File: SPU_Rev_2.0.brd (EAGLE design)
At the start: 141 x 101.6 mm, 139 parts, among them Q1 12MHz

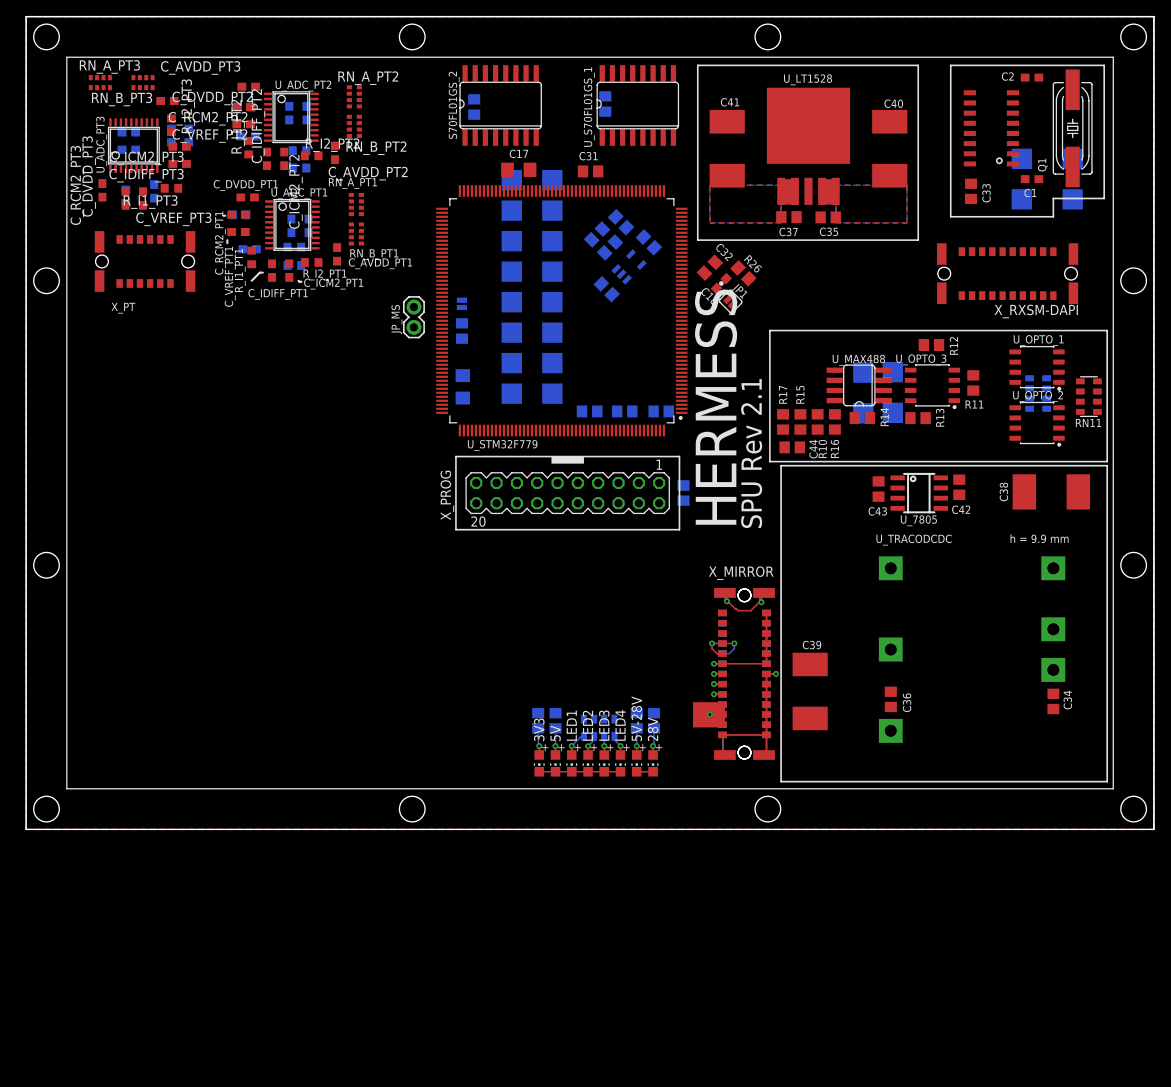
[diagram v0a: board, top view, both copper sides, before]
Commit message: rev 2.1
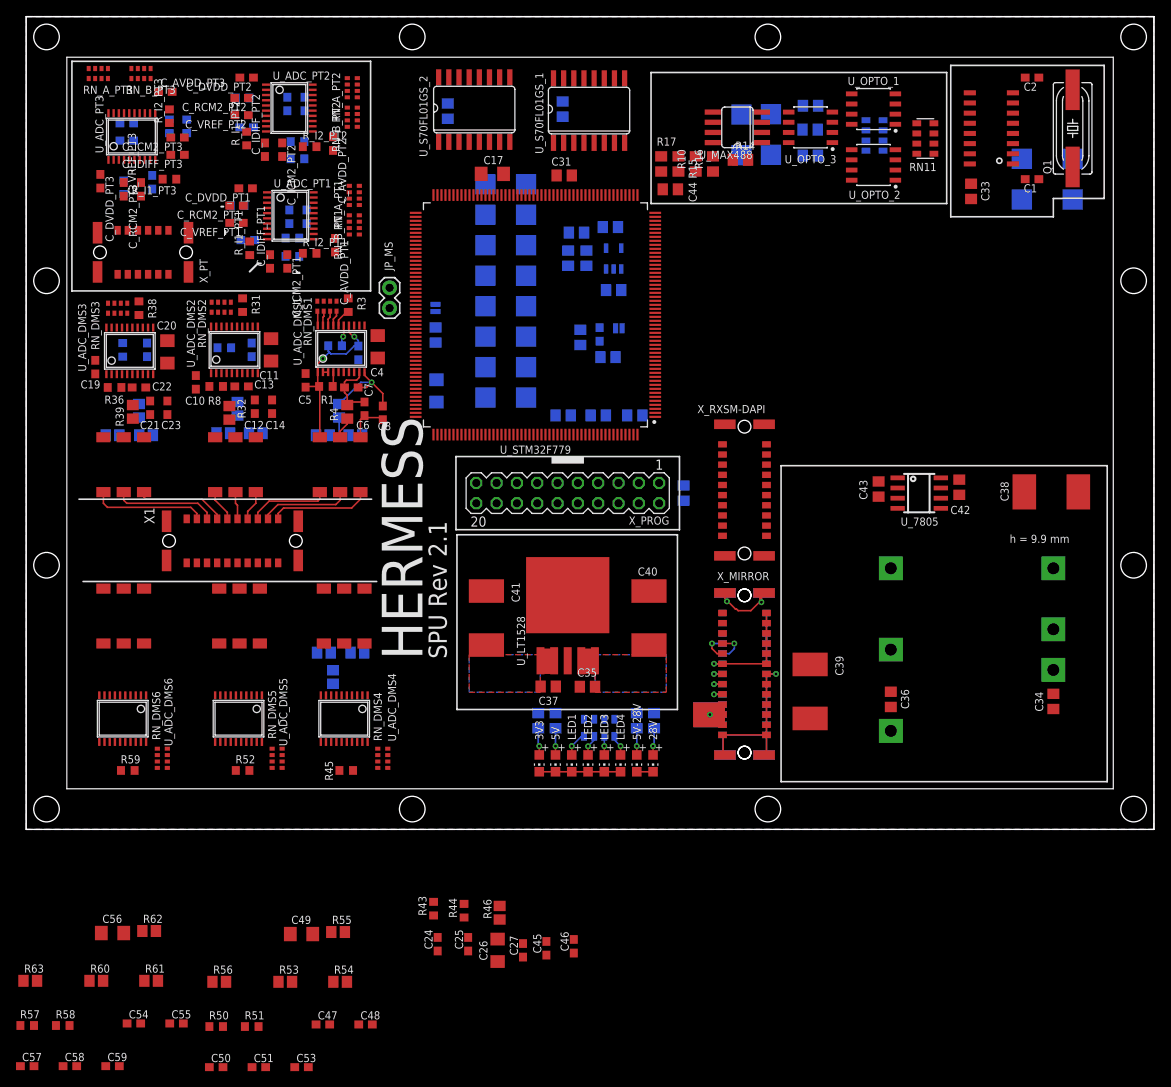
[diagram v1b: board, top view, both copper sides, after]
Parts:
- removed S70FL01GS_2: S70FL01GS, S70FL01GS:SO16
- added C10, C12, C13, C14, C15, C19, C21, C22, C23, C24, C25, C27, C3, C45, C46, C47, C48, C5, C50, C51, C53, C54, C55, C57, C58, C59, C6, C7, C8, C9: 100n, rcl:C0603
- added C11, C20, C26, C4, C49, C56: 1u, rcl:C1206
- added R1, R2, R30, R36, R37, R43, R44, R50, R51, R57, R58, R8: 4k7, ++Bedrahtet:R0603
- added R3, R31, R38, R45, R52, R59: 47, ++Bedrahtet:R0603
- added R32, R33, R39, R4, R40, R46, R47, R5, R53, R54, R60, R61: 40 1%, ++Bedrahtet:R0805
- added R34, R35, R41, R42, R48, R49, R55, R56, R6, R62, R63, R7: 1k 0.1%, ++Bedrahtet:R0805
- added RN_DMS1, RN_DMS2, RN_DMS3, RN_DMS4, RN_DMS5, RN_DMS6: 47, resistor-dil:0603-ARC
- added U$1, U$2, U$3, U$4, U$5, U$6: COMMON_MODE_CHOKE, selfmade:COMMON_MODE_CHOKE
- added U_ADC_DMS1, U_ADC_DMS2, U_ADC_DMS3, U_ADC_DMS4, U_ADC_DMS5, U_ADC_DMS6: ADS1147TSSOP20, ads11xx:TSSOP20
- added U_S70FL01GS_2: S70FL01GS, S70FL01GS:SO16
- added X1: 403-5X020-5X, con-ept-One27:403-5X020-5X
- moved C40 65.9 mm to (82.9, 26.4)
- moved C41 65.9 mm to (62.6, 26.4)
- moved C35 65.9 mm to (75.2, 17.8)
- moved C37 65.9 mm to (70.3, 17.9)
- moved U_LT1528 65.9 mm to (72.8, 29.0)
- moved X_RXSM-DAPI 42.6 mm to (94.9, 42.4), turned to 270 degrees
- moved RN11 38.2 mm to (117.5, 86.4)
- moved RN12 38.2 mm to (111.1, 86.7)
- moved U_OPTO_1 38.2 mm to (111.0, 90.0)
- moved U_OPTO_2 38.2 mm to (111.0, 83.1)
- moved R11 37.7 mm to (103.1, 87.5), flipped to the bottom, turned to 180 degrees
- moved R10 35.7 mm to (88.8, 83.2)
- moved U_OPTO_3 35.7 mm to (103.1, 87.8)
- moved C44 35.7 mm to (85.6, 80.0)
- moved D5 35.7 mm to (98.2, 86.9)
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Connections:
- net PT1_DIN renamed PT_DIN
- net PT1_DOUT renamed PT_DOUT
- net PT1_SCLK renamed PT_SCLK
- removed net PT1_!CS: RN_B_PT1.7, RN_B_PT2.7, RN_B_PT3.7
- removed net PT1_!DRDY: RN_B_PT1.8, RN_B_PT2.8, RN_B_PT3.8
- removed net PT1_!RESET: RN_A_PT1.8, RN_A_PT2.8, RN_A_PT3.8
- removed net PT1_START: RN_B_PT1.6, RN_B_PT2.6, RN_B_PT3.6
- new net !CS!_DMS1: R3.2
- new net !CS!_DMS2: R31.2
- new net !CS!_DMS3: R38.2
- new net !CS!_DMS4: R45.2
- new net !CS!_DMS5: R52.2
- new net !CS!_DMS6: R59.2
- new net !CS!_PT1: RN_B_PT1.7
- new net !CS!_PT2: RN_B_PT2.7
- new net !CS!_PT3: RN_B_PT3.7
- new net !DRDY!_DMS1: RN_DMS1.5
- new net !DRDY!_DMS2: RN_DMS2.5
- new net !DRDY!_DMS3: RN_DMS3.5
- new net !DRDY!_DMS4: RN_DMS4.5
- new net !DRDY!_DMS5: RN_DMS5.5
- new net !DRDY!_DMS6: RN_DMS6.5
- new net !DRDY!_PT1: RN_B_PT1.8
- new net !DRDY!_PT2: RN_B_PT2.8
- new net !DRDY!_PT3: RN_B_PT3.8
- new net DMS11: U$2.P$1, X1.P$B3
- new net DMS12: U$2.P$3, X1.P$B2
- new net DMS13: U$2.P$5, X1.P$B1
- new net DMS21: U$1.P$1, X1.P$B6
- new net DMS22: U$1.P$3, X1.P$B5
- new net DMS23: U$1.P$5, X1.P$B4
- new net DMS31: U$3.P$1, X1.P$B9
- new net DMS32: U$3.P$3, X1.P$B8
- new net DMS33: U$3.P$5, X1.P$B7
- new net DMS41: U$4.P$1, X1.P$A1
- new net DMS42: U$4.P$3, X1.P$A2
- new net DMS43: U$4.P$5, X1.P$A3
- new net DMS51: U$5.P$1, X1.P$A4
- new net DMS52: U$5.P$3, X1.P$A5
- new net DMS53: U$5.P$5, X1.P$A6
- new net DMS61: U$6.P$1, X1.P$A7
- new net DMS62: U$6.P$3, X1.P$A8
- new net DMS63: U$6.P$5, X1.P$A9
- new net DMS_DIN: RN_DMS1.7, RN_DMS2.7, RN_DMS3.7, RN_DMS4.7, RN_DMS5.7, RN_DMS6.7
- new net DMS_DOUT: RN_DMS1.6, RN_DMS2.6, RN_DMS3.6, RN_DMS4.6, RN_DMS5.6, RN_DMS6.6
- new net DMS_SCLK: RN_DMS1.8, RN_DMS2.8, RN_DMS3.8, RN_DMS4.8, RN_DMS5.8, RN_DMS6.8
- new net N$10: RN_DMS1.1, U_ADC_DMS1.20
- new net N$100: RN_DMS3.4, U_ADC_DMS3.17
- new net N$101: R38.1, U_ADC_DMS3.16
- new net N$102: C27.2, C45.1, R46.1, U_ADC_DMS4.9
- new net N$103: C45.2, C46.1, R47.1, U_ADC_DMS4.10
- new net N$104: R47.2, R48.1, R49.1
- new net N$105: C26.1, U_ADC_DMS4.7
- new net N$106: R46.2, U$4.P$4
- new net N$107: R43.2, U_ADC_DMS4.4
- new net N$108: R44.1, U_ADC_DMS4.15
- new net N$109: RN_DMS4.1, U_ADC_DMS4.20
- new net N$11: C13.2, C14.1, R33.1, U_ADC_DMS2.10
- new net N$110: RN_DMS4.2, U_ADC_DMS4.19
- new net N$111: RN_DMS4.3, U_ADC_DMS4.18
- new net N$112: RN_DMS4.4, U_ADC_DMS4.17
- new net N$113: R45.1, U_ADC_DMS4.16
- new net N$114: C50.2, C51.1, R53.1, U_ADC_DMS5.9
- new net N$115: C51.2, C53.1, R54.1, U_ADC_DMS5.10
- new net N$116: R54.2, R55.1, R56.1
- new net N$117: C49.1, U_ADC_DMS5.7
- new net N$118: R53.2, U$5.P$4
- new net N$119: R50.2, U_ADC_DMS5.4
- new net N$12: R33.2, R34.1, R35.1
- new net N$120: R51.1, U_ADC_DMS5.15
- new net N$121: RN_DMS5.1, U_ADC_DMS5.20
- new net N$122: RN_DMS5.2, U_ADC_DMS5.19
- new net N$123: RN_DMS5.3, U_ADC_DMS5.18
- new net N$124: RN_DMS5.4, U_ADC_DMS5.17
- new net N$125: R52.1, U_ADC_DMS5.16
- new net N$127: C47.1, R50.1, U_ADC_DMS5.1
- new net N$128: C57.2, C58.1, R60.1, U_ADC_DMS6.9
- new net N$129: C58.2, C59.1, R61.1, U_ADC_DMS6.10
- new net N$130: R61.2, R62.1, R63.1
- new net N$131: C56.1, U_ADC_DMS6.7
- new net N$132: R60.2, U$6.P$4
- new net N$133: R57.2, U_ADC_DMS6.4
- new net N$134: R58.1, U_ADC_DMS6.15
- new net N$135: RN_DMS6.1, U_ADC_DMS6.20
- new net N$136: RN_DMS6.2, U_ADC_DMS6.19
- new net N$137: RN_DMS6.3, U_ADC_DMS6.18
- new net N$138: RN_DMS6.4, U_ADC_DMS6.17
- new net N$139: R59.1, U_ADC_DMS6.16
- new net N$141: C54.1, R57.1, U_ADC_DMS6.1
- new net N$148: X1.P$B10
- new net N$157: X1.P$A10
- new net N$2: R2.1, U_ADC_DMS1.15
- new net N$67: C11.1, U_ADC_DMS2.7
- new net N$7: C12.2, C13.1, R32.1, U_ADC_DMS2.9
- new net N$72: R32.2, U$1.P$4
- new net N$73: R1.2, U_ADC_DMS1.4
- new net N$74: RN_DMS1.2, U_ADC_DMS1.19
- new net N$75: RN_DMS1.3, U_ADC_DMS1.18
- new net N$76: RN_DMS1.4, U_ADC_DMS1.17
- new net N$77: R3.1, U_ADC_DMS1.16
- new net N$78: R8.2, U_ADC_DMS2.4
- new net N$79: R30.1, U_ADC_DMS2.15
- new net N$80: C6.2, C7.1, R4.1, U_ADC_DMS1.9
- new net N$81: C7.2, C8.1, R5.1, U_ADC_DMS1.10
- new net N$82: R5.2, R6.1, R7.1
- new net N$83: C4.1, U_ADC_DMS1.7
- new net N$84: R4.2, U$2.P$4
- new net N$85: RN_DMS2.1, U_ADC_DMS2.20
- new net N$86: RN_DMS2.2, U_ADC_DMS2.19
- new net N$87: RN_DMS2.3, U_ADC_DMS2.18
- new net N$88: RN_DMS2.4, U_ADC_DMS2.17
- new net N$89: R31.1, U_ADC_DMS2.16
- new net N$90: C21.2, C22.1, R39.1, U_ADC_DMS3.9
- new net N$91: C22.2, C23.1, R40.1, U_ADC_DMS3.10
- new net N$92: R40.2, R41.1, R42.1
- new net N$93: C20.1, U_ADC_DMS3.7
- new net N$94: R39.2, U$3.P$4
- new net N$95: R36.2, U_ADC_DMS3.4
- new net N$96: R37.1, U_ADC_DMS3.15
- new net N$97: RN_DMS3.1, U_ADC_DMS3.20
- new net N$98: RN_DMS3.2, U_ADC_DMS3.19
- new net N$99: RN_DMS3.3, U_ADC_DMS3.18
- net 3V3: now also C10.1, C15.1, C19.1, C24.1, C25.1, C3.1, C48.1, C5.1, C55.1, C9.1, R1.1, R2.2, R30.2, R34.2, R36.1, R37.2, R41.2, R43.1, R44.2, R48.2, R51.2, R55.2, R58.2, R6.2, R62.2, R8.1, RN_A_PT1.8, RN_A_PT2.8, RN_A_PT3.8, RN_B_PT1.6, RN_B_PT2.6, RN_B_PT3.6, U$1.P$2, U$2.P$2, U$3.P$2, U$4.P$2, U$5.P$2, U$6.P$2, U_ADC_DMS1.1, U_ADC_DMS1.14, U_ADC_DMS2.1, U_ADC_DMS2.14, U_ADC_DMS3.1, U_ADC_DMS3.14, U_ADC_DMS4.1, U_ADC_DMS4.14, U_ADC_DMS5.14, U_ADC_DMS6.14, U_S70FL01GS_2.2; no longer S70FL01GS_2.2
- net FL_2_CS1: now also U_S70FL01GS_2.7; no longer S70FL01GS_2.7
- net FL_2_CS2: now also U_S70FL01GS_2.6; no longer S70FL01GS_2.6
- net FL_2_HLD: now also U_S70FL01GS_2.1; no longer S70FL01GS_2.1
- net FL_2_RES: now also U_S70FL01GS_2.3; no longer S70FL01GS_2.3
- net FL_2_WP: now also U_S70FL01GS_2.9; no longer S70FL01GS_2.9
- net GND: now also C10.2, C11.2, C12.1, C14.2, C15.2, C19.2, C20.2, C21.1, C23.2, C24.2, C25.2, C26.2, C27.1, C3.2, C4.2, C46.2, C47.2, C48.2, C49.2, C5.2, C50.1, C53.2, C54.2, C55.2, C56.2, C57.1, C59.2, C6.1, C8.2, C9.2, R35.2, R42.2, R49.2, R56.2, R63.2, R7.2, U$1.P$6, U$2.P$6, U$3.P$6, U$4.P$6, U$5.P$6, U$6.P$6, U_ADC_DMS1.13, U_ADC_DMS1.2, U_ADC_DMS1.3, U_ADC_DMS1.8, U_ADC_DMS2.13, U_ADC_DMS2.2, U_ADC_DMS2.3, U_ADC_DMS2.8, U_ADC_DMS3.13, U_ADC_DMS3.2, U_ADC_DMS3.3, U_ADC_DMS3.8, U_ADC_DMS4.13, U_ADC_DMS4.2, U_ADC_DMS4.3, U_ADC_DMS4.8, U_ADC_DMS5.13, U_ADC_DMS5.2, U_ADC_DMS5.3, U_ADC_DMS5.8, U_ADC_DMS6.13, U_ADC_DMS6.2, U_ADC_DMS6.3, U_ADC_DMS6.8, U_S70FL01GS_2.10; no longer S70FL01GS_2.10
- net SPI2_MISO: now also U_S70FL01GS_2.8; no longer S70FL01GS_2.8
- net SPI2_MOSI: now also U_S70FL01GS_2.15; no longer S70FL01GS_2.15
- net SPI2_SCK: now also U_S70FL01GS_2.16; no longer S70FL01GS_2.16
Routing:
- net 3V3: track 0.00 -> 21.2 mm, vias 0 -> 2
- net DMS31: track 0.00 -> 14.3 mm
- net DMS32: track 0.00 -> 12.9 mm
- net DMS13: track 0.00 -> 12.6 mm
- net N$81: track 0.00 -> 12.3 mm, vias 0 -> 1
- net DMS12: track 0.00 -> 11.3 mm
- net DMS33: track 0.00 -> 11.2 mm
- net DMS11: track 0.00 -> 10.1 mm
- net N$80: track 0.00 -> 8.08 mm
- net GND: track 31.7 -> 37.8 mm
- net N$82: track 0.00 -> 4.56 mm
- net DMS21: track 0.00 -> 3.98 mm
- net DMS23: track 0.00 -> 3.77 mm
- net DMS22: track 0.00 -> 3.45 mm
- net N$84: track 0.00 -> 2.69 mm
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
